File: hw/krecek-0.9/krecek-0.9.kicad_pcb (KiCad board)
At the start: 4 copper layers, 177.8 x 88.9 mm, 174 parts, among them CN1 PJ-313B6-B, J1 DAP, J2 AUX, J3 USB_C_Receptacle_USB2.0, J4 U.FL, J5 Micro_SD_Card_Det1, Q1 AO3401A, Q2 AO3401A, Q3 AO3400A, Q4 AO3400A, Q5 AO3400A, Q6 AO3400A, Q7 PT334, Q8 AO3400A, SW1 SW_Push, SW5 TM-2023, U1 Display, U10 TPS63000, U11 ES8312, U13 CC1101RGPR, U14 PAM8302AASCR, U2 RP2040, U3 RP2040, U4 W25Q128JVS, U5 AMS1117-3.3, U6 JST-PH-2P, U7 BQ24040DSQR, U8 AMS1117-3.3, U9 AMS1117-3.3, Y1 12MHz

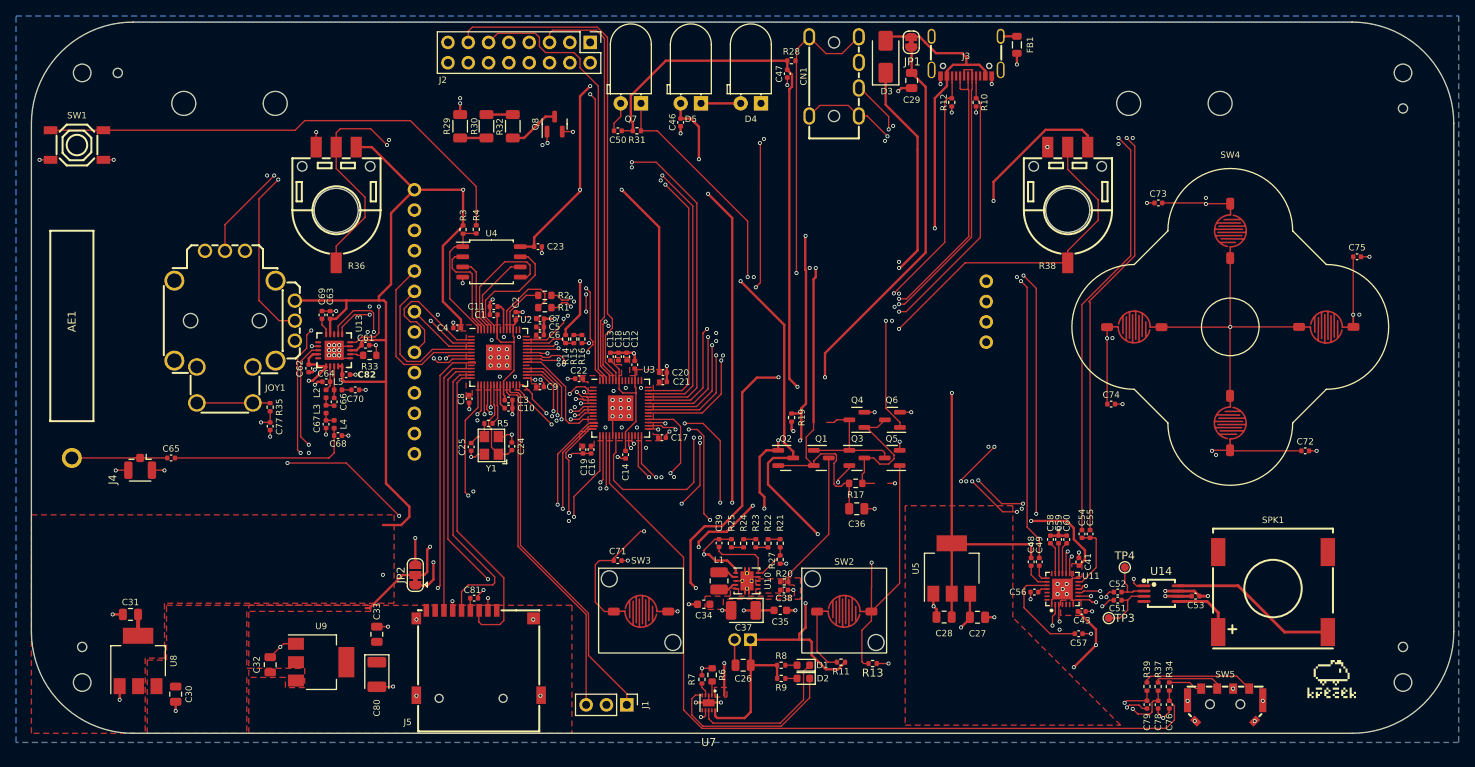
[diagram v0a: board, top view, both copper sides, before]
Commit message: Use display without PCB
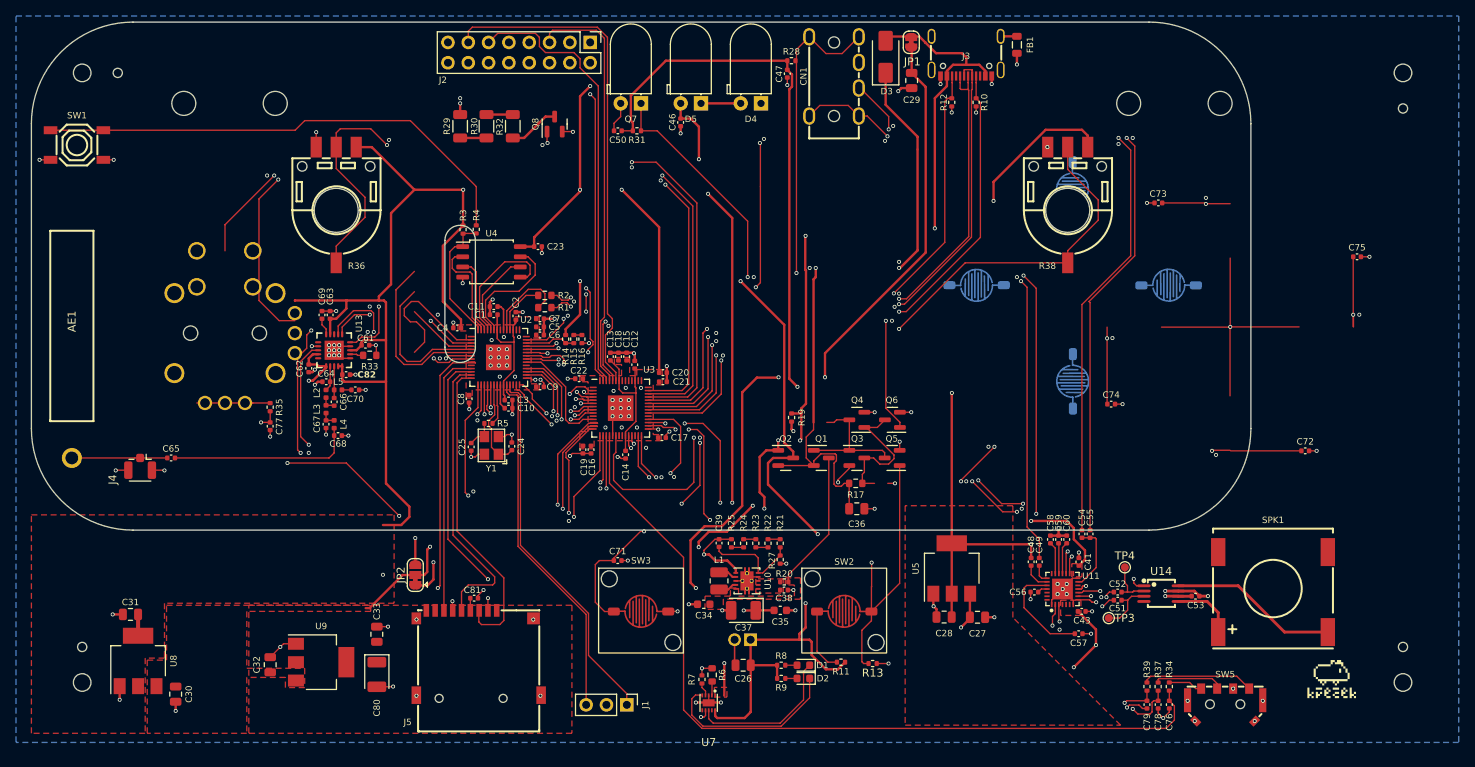
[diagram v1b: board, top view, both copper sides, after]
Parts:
- removed U1: Display, Krecek:TftDisplay
- added REF**: Panel, Krecek:Panel, B.Cu at (126.0, 71.1)
- JOY1, SW4: moved to B.Cu
- moved SW4 20.4 mm to (181.0, 71.0), turned to 180 degrees
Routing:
- net /Inputs/BTN_{Y}: track 0.00 -> 92.4 mm, vias 0 -> 2
- net /RP2040/TFT_{LED}: track 75.1 -> 0.00 mm, vias 3 -> 0
- net /RP2040/AUX4: track 52.0 -> 127.1 mm, vias 0 -> 3
- net /Inputs/BTN_{B}: track 181.9 -> 108.5 mm, vias 4 -> 2
- net /Inputs/BTN_{X}: track 92.4 -> 73.4 mm
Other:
- board size 177.8 x 88.9 mm -> 152.4 x 63.5 mm
